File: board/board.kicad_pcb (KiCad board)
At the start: 2 copper layers, 45 x 13 mm, 34 parts, among them J1 Conn_01x02_Pin, J2 Conn_01x02_Pin, J3 003_power, U1 TPS65131

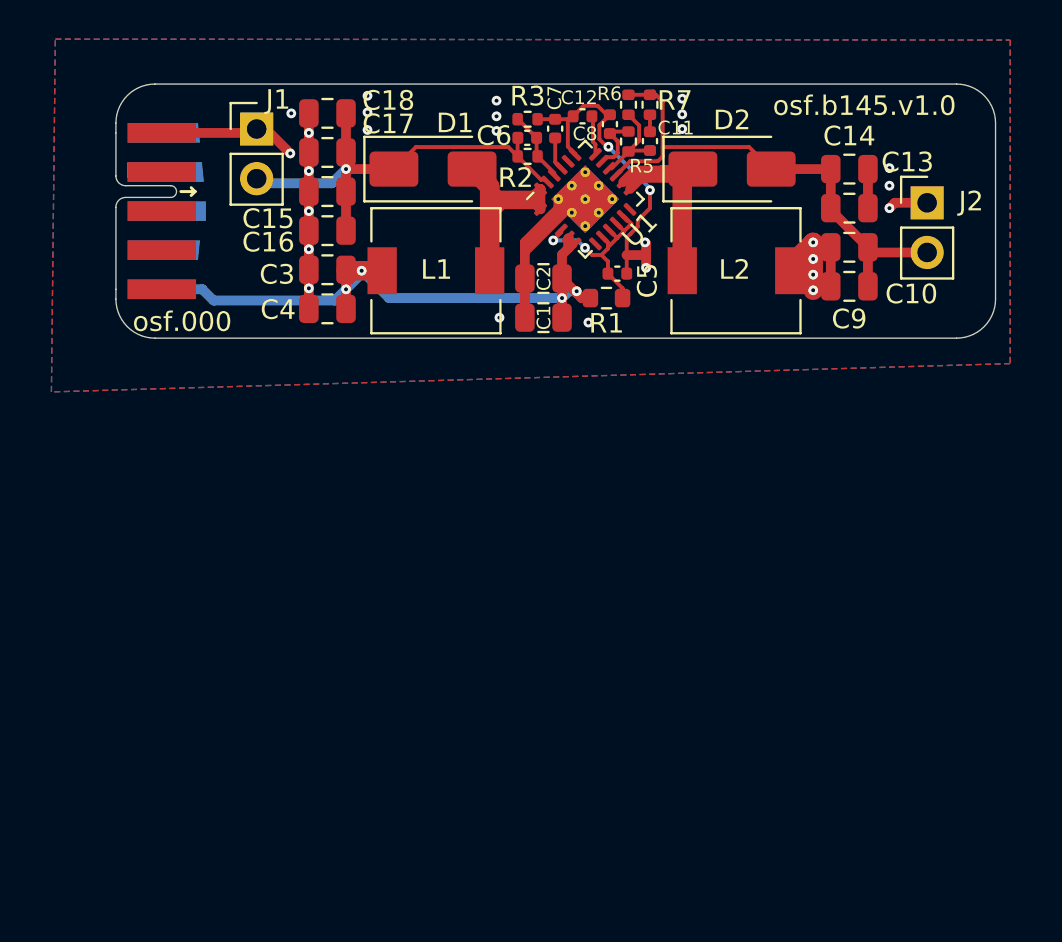
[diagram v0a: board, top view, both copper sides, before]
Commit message: initial b147
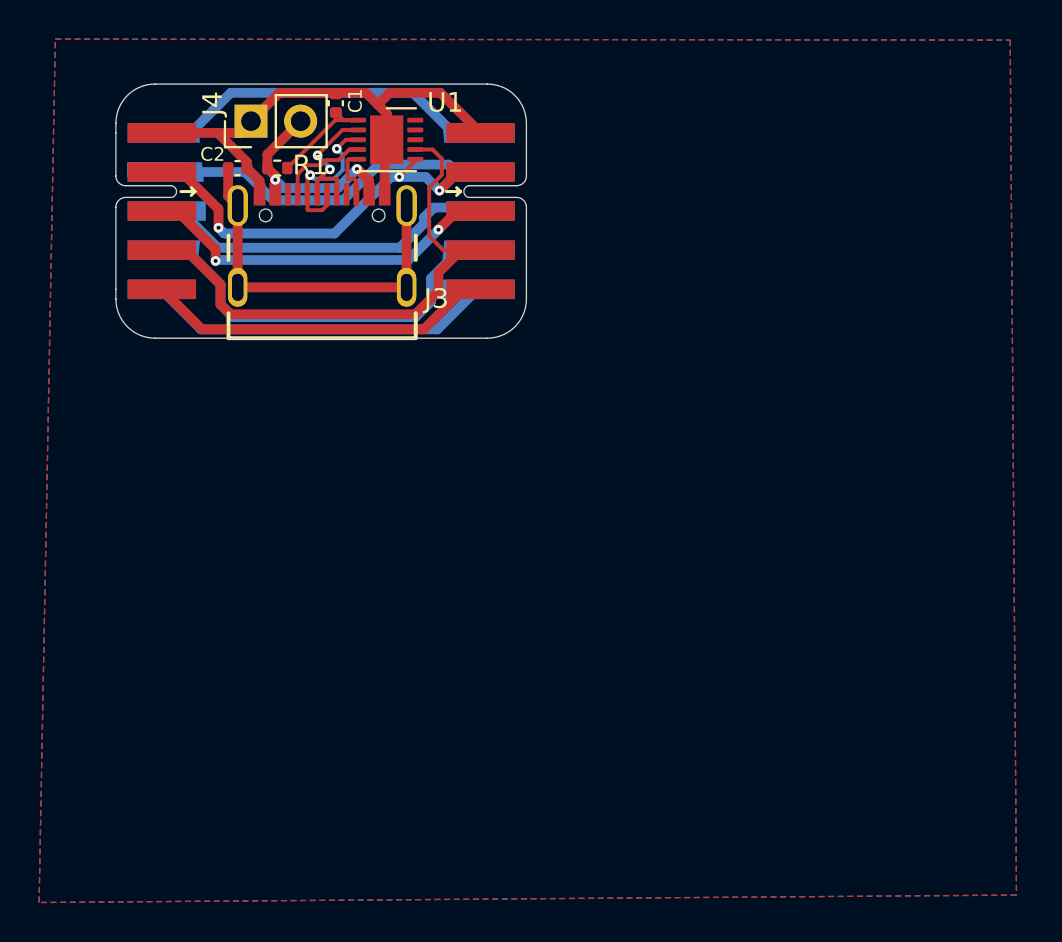
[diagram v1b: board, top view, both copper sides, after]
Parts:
- removed C10, C13, C14, C15, C16, C17, C18, C3, C4, C9: 22uF, Capacitor_SMD:C_0805_2012Metric
- removed C11, C6: 10pF, Capacitor_SMD:C_0402_1005Metric
- removed C12: 220nF, Capacitor_SMD:C_0402_1005Metric
- removed C5: 100nF, Capacitor_SMD:C_0402_1005Metric
- removed C7: 10nF, Capacitor_SMD:C_0402_1005Metric
- removed C8: 4.7nF, Capacitor_SMD:C_0402_1005Metric
- removed D1, D2: SS12, Diode_SMD:D_SMA
- removed L1, L2: 4.7uH, Inductor_SMD:L_6.3x6.3_H3
- removed NT1: NetTie_2, NetTie:NetTie-2_SMD_Pad0.5mm
- removed R2, R6: 1M, Resistor_SMD:R_0402_1005Metric
- removed R3: 100k, Resistor_SMD:R_0402_1005Metric
- removed R5: 82k, Resistor_SMD:R_0402_1005Metric
- removed R7: 51k, Resistor_SMD:R_0402_1005Metric
- added J4: Conn_01x02_Pin, Connector_PinHeader_2.54mm:PinHeader_1x02_P2.54mm_Vertical, F.Cu at (146.9, 91.9)
- C1: value 22uF -> 1uF; footprint Capacitor_SMD:C_0805_2012Metric -> Capacitor_SMD:C_0402_1005Metric
- C2: value 22uF -> 100pF; footprint Capacitor_SMD:C_0805_2012Metric -> Capacitor_SMD:C_0402_1005Metric
- J1: value Conn_01x02_Pin -> 001_I2C; footprint Connector_PinHeader_2.54mm:PinHeader_1x02_P2.54mm_Vertical -> on_edge:on_edge_2x05_host
- J2: value Conn_01x02_Pin -> 001_I2C; footprint Connector_PinHeader_2.54mm:PinHeader_1x02_P2.54mm_Vertical -> on_edge:on_edge_2x05_device
- J3: value 003_power -> USB4105-GF-A; footprint on_edge:on_edge_2x05_device -> b051:GCT_USB4105-GF-A
- R1: value 100R -> 10R; footprint Resistor_SMD:R_0603_1608Metric -> Resistor_SMD:R_0402_1005Metric
- U1: value TPS65131 -> HUSB238; footprint Package_DFN_QFN:VQFN-24-1EP_4x4mm_P0.5mm_EP2.45x2.45mm_ThermalVias -> Package_DFN_QFN:DFN-10-1EP_3x3mm_P0.5mm_EP1.7x2.5mm
- moved J2 41.5 mm to (140.0, 96.5), turned to -90 degrees
- moved R1 18.1 mm to (148.3, 94.3)
- moved C2 16.6 mm to (146.2, 94.3), turned to 0 degrees
- moved C1 15.3 mm to (151.2, 91.0), turned to 90 degrees
- moved J1 14.4 mm to (161.0, 96.5), turned to -90 degrees
- moved J3 11.2 mm to (150.6, 100.4), turned to 0 degrees
- moved U1 10.6 mm to (153.8, 92.8), turned to 0 degrees
- moved LOGO1 5.78 mm to (150.6, 97.6)
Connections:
- C1 pad 1: /DCDC/5V -> Net-(U1-VIN)
- C2 pad 1: /DCDC/5V -> Net-(C2-Pad1)
- J1 pad 2: /DCDC/+out -> /USB_PD/SDA
- J2 pad 2: /DCDC/-out -> /USB_PD/SDA
- R1 pad 1: /DCDC/5V -> /USB_PD/VBUS
- R1 pad 2: Net-(U1-ENN) -> Net-(U1-VIN)
- U1 pad 1: Net-(D1-A) -> Net-(U1-VIN)
- U1 pad 10: Net-(U1-ENN) -> /USB_PD/GATE
- U1 pad 11: Net-(U1-ENN) -> GND
- U1 pad 2: GND -> /USB_PD/D+
- U1 pad 3: GND -> /USB_PD/D-
- U1 pad 4: Net-(U1-ENN) -> /USB_PD/CC1
- U1 pad 5: /DCDC/5V -> /USB_PD/CC2
- U1 pad 6: /DCDC/5V -> /USB_PD/SDA
- U1 pad 7: unconnected-(U1-BSW-Pad7) -> /USB_PD/SCL
- U1 pad 8: Net-(U1-ENN) -> /USB_PD/VSET
- U1 pad 9: Net-(U1-ENN) -> /USB_PD/ISET
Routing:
- net /DCDC/5V: track 35.1 -> 0.00 mm, vias 4 -> 0
- net /USB_PD/SCL: track 0.00 -> 28.9 mm
- net /DCDC/-out: track 26.7 -> 0.00 mm
- net /DCDC/+out: track 24.3 -> 0.00 mm, vias 1 -> 0
- net /USB_PD/SDA: track 0.00 -> 21.3 mm, vias 0 -> 3
- net Net-(J1-3.3V): track 0.00 -> 20.3 mm
- net Net-(C2-Pad1): track 0.00 -> 19.1 mm
- net Net-(J1-SCL): track 0.00 -> 18.8 mm, vias 0 -> 2
- net Net-(J1-status): track 0.00 -> 18.1 mm
- net Net-(J1-INT): track 0.00 -> 18.0 mm
- net Net-(J1-~{RESET}): track 0.00 -> 17.9 mm
- net Net-(J1-5V): track 0.00 -> 17.9 mm
- net Net-(J1-CS/EN): track 0.00 -> 17.9 mm
- net Net-(D1-A): track 17.9 -> 0.00 mm
- net Net-(D2-K): track 17.3 -> 0.00 mm
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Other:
- board size 45 x 13 mm -> 21 x 13 mm
- board text added: "osf.b147.v1.0"
- board text removed: "osf.000"
- board text removed: "osf.b145.v1.0"
